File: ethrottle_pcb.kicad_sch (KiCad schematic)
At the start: 49 parts

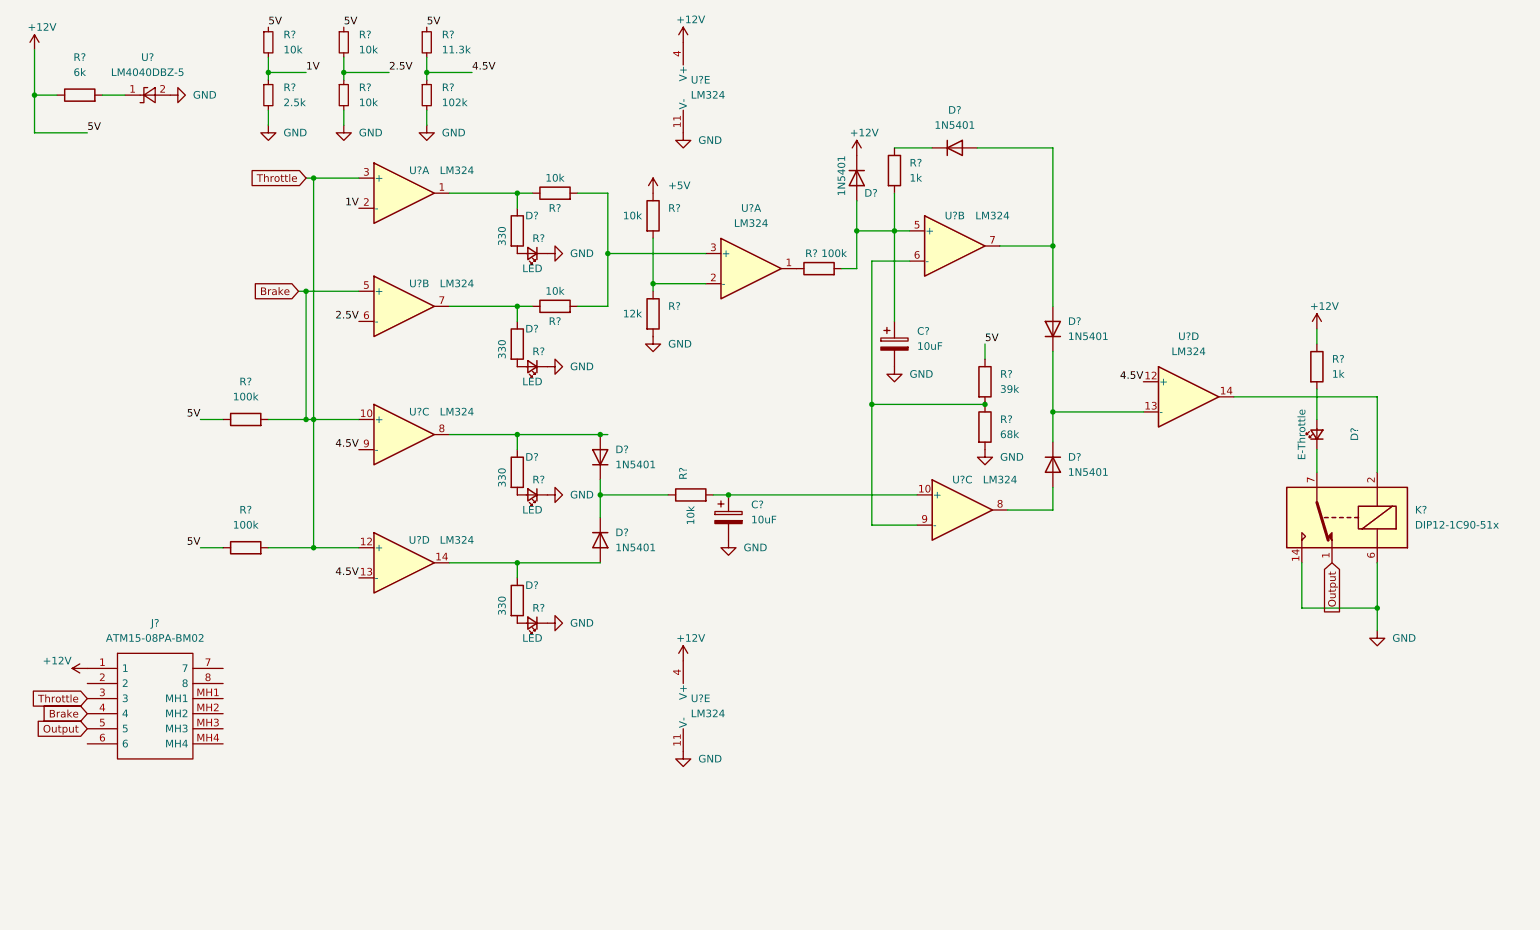
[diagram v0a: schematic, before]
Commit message: layout in progress
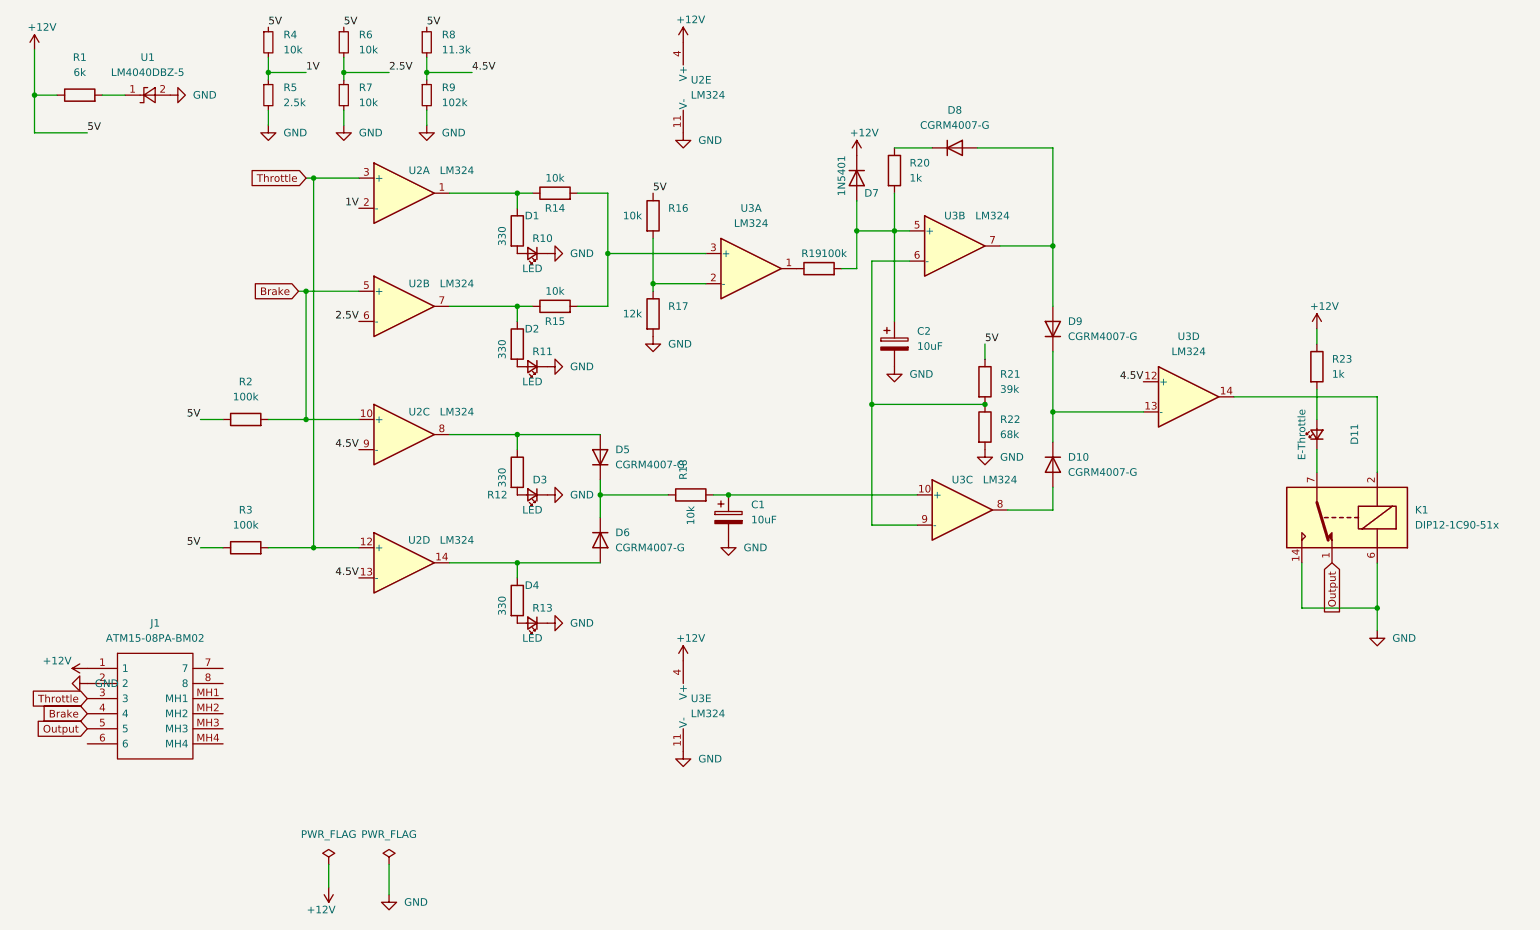
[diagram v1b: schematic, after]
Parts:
- D1, D11, D2, D3, D4: renamed from D?; footprint APGF0606SYKCGK-TT-C2:APGF0606SYKCGKTTC2 -> LED_SMD:LED_0402_1005Metric
- D10, D5, D6, D8, D9: renamed from D?; value 1N5401 -> CGRM4007-G; footprint Diode_THT:D_DO-201AD_P15.24mm_Horizontal -> Diode_SMD:D_SOD-123
- U2, U3: renamed from U?; footprint LM324N_NOPB:DIP825W47P254L1917H533Q14 -> LM324PWR:LM324PWR
- U2, U3: renamed from U?; footprint (none) -> LM324PWR:LM324PWR
- gave numbers to parts that had none: 29
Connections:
- net +5V is gone; now on net +12V: R16.1
- net Brake: no longer J1.3, R3.2, U2.12 (+), U2.3 (+)
- net GND: now also J1.2
- new net Throttle: J1.3, R3.2, U2.12 (+), U2.3 (+)
